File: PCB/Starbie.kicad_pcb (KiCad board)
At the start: 2 copper layers, 96.6 x 82.8 mm, 11 parts, among them J1 Conn_01x04_Pin, J2 Conn_01x08_Pin, SW1 SW_Push, SW2 SW_Push, U1 DHT11, U2 XIAO-ESP32-C3-SMD

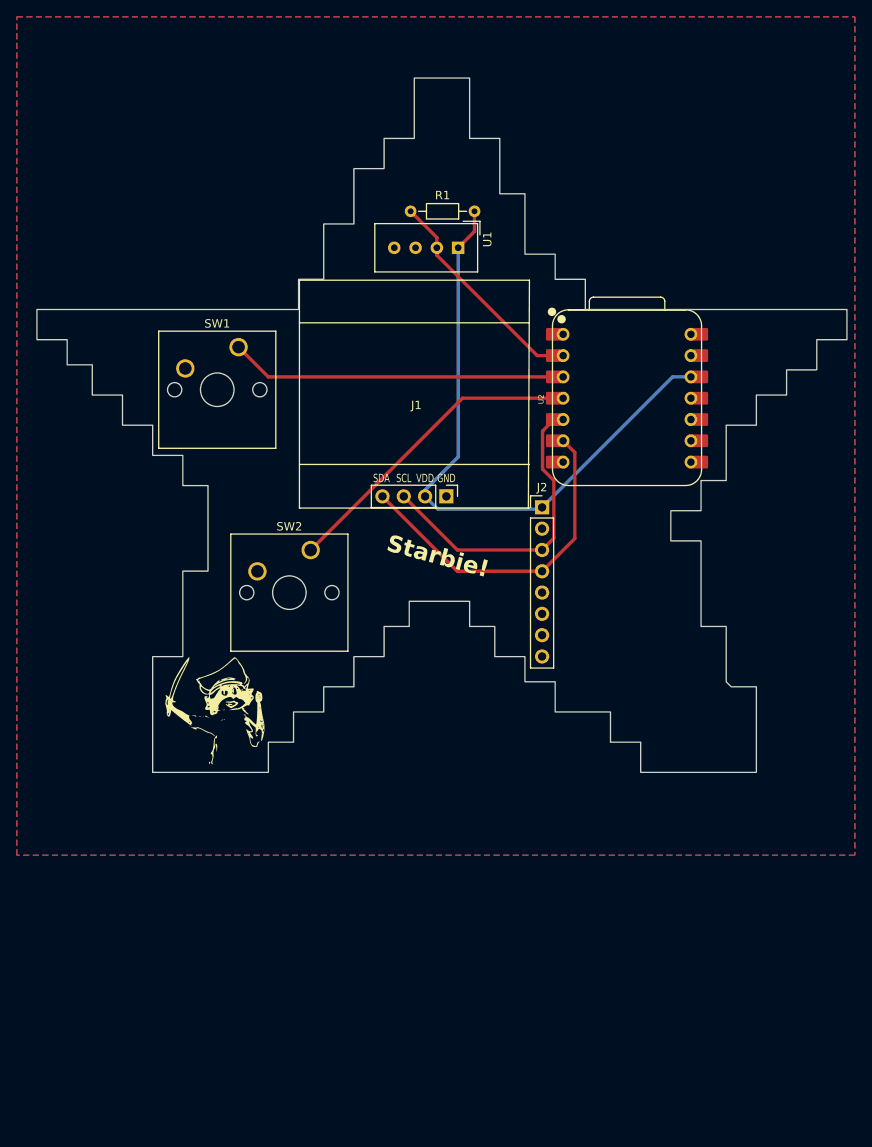
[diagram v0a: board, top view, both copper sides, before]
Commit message: Update Starbie guide images, BOM, and PCB layout
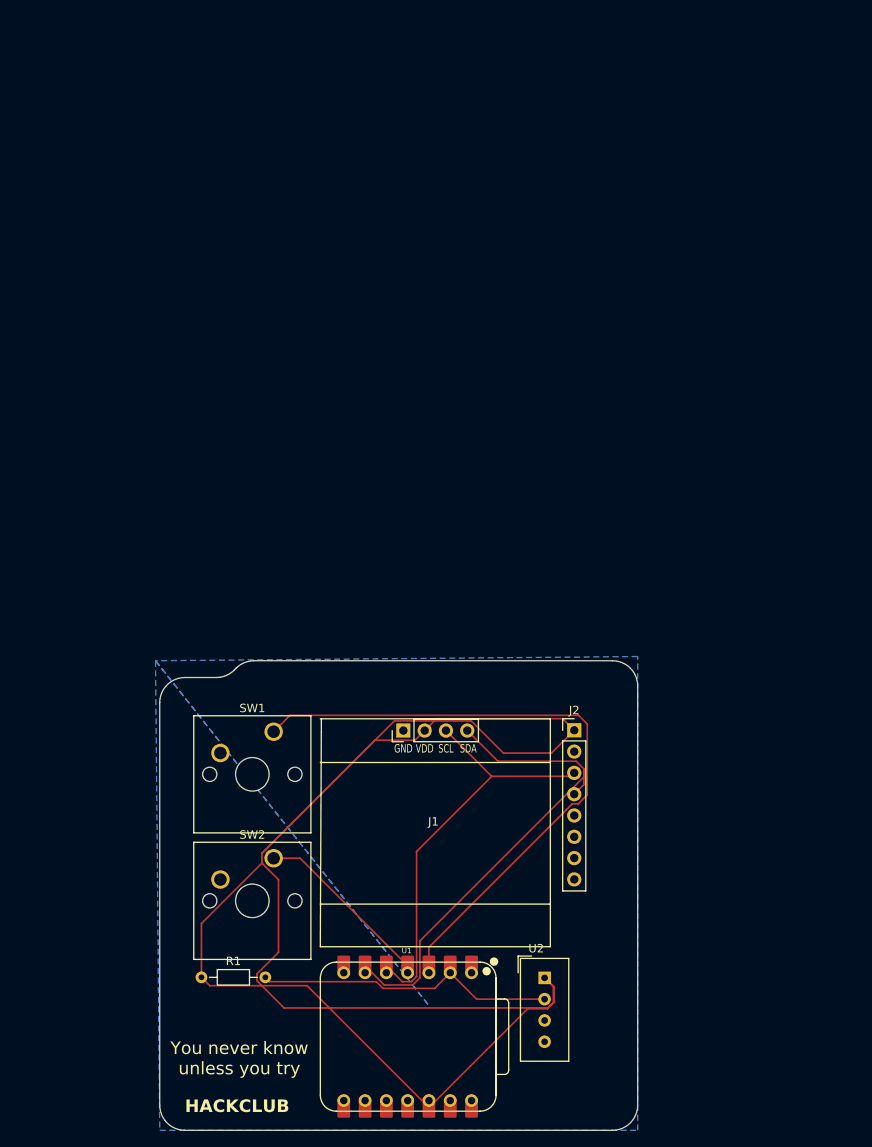
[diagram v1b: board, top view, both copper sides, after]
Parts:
- removed the G*** at (118.9, 71.9)
- removed the G*** at (92.8, 104.0)
- removed the G*** at (113.0, 89.6)
- removed the G*** at (113.0, 64.6)
- added G***: LOGO, cute_dragon_cat_debanjan_bsilk, F.Cu at (117.9, 122.0)
- U1: value DHT11 -> XIAO-ESP32-C3-SMD; footprint Sensor:Aosong_DHT11_5.5x12.0_P2.54mm -> Imported Parts:XIAO-ESP32-C6-DIP
- U2: value XIAO-ESP32-C3-SMD -> DHT11; footprint Imported Parts:XIAO-ESP32-C6-DIP -> Sensor:Aosong_DHT11_5.5x12.0_P2.54mm
- moved R1 97.0 mm to (90.0, 137.8), turned to 0 degrees
- moved U1 94.3 mm to (114.6, 144.8), turned to 0 degrees
- moved U2 69.8 mm to (130.9, 137.8), turned to 0 degrees
- moved SW1 46.1 mm to (98.6, 108.5)
- moved SW2 37.0 mm to (98.6, 123.6)
- moved J1 28.0 mm to (117.9, 108.3), turned to 0 degrees
- moved J2 26.9 mm to (134.4, 108.3)
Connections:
- U1 pad 1: +3.3V -> unconnected-(U1-D0-Pad1)_1
- U1 pad 3: unconnected-(U1-NC-Pad3) -> /GPIO2
- U1 pad 4: GND -> /GPIO3
- U2 pad 1: unconnected-(U2-D0-Pad1) -> +3.3V
- U2 pad 3: /GPIO2 -> unconnected-(U2-NC-Pad3)
- U2 pad 4: /GPIO3 -> GND
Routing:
- net +3.3V: track 75.3 -> 222.1 mm
- net /GPIO2: track 40.2 -> 76.5 mm
- net /SDA: track 40.5 -> 60.2 mm
- net /GPIO3: track 37.6 -> 21.3 mm
- net /SCL: track 37.5 -> 50.0 mm
- net /DHT11 DATA: track 26.6 -> 35.9 mm
- removed copper zone on F.Cu, net GND
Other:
- board size 96.6 x 82.8 mm -> 57 x 56 mm
- board text added: "HACKCLUB"
- board text added: "You never know unless you try"
- board text removed: "Designed By Logan Peterson"
- board text removed: "Starbie!"
